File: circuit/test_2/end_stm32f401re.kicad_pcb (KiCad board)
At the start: 2 copper layers, 70 x 55.8 mm, 37 parts, among them J1 Micro_SD_Card_Det, J2 USB_B_Micro, U1 MAX98357_DAC, U2 STM32F401RETx, U3 AMS1117-3.3

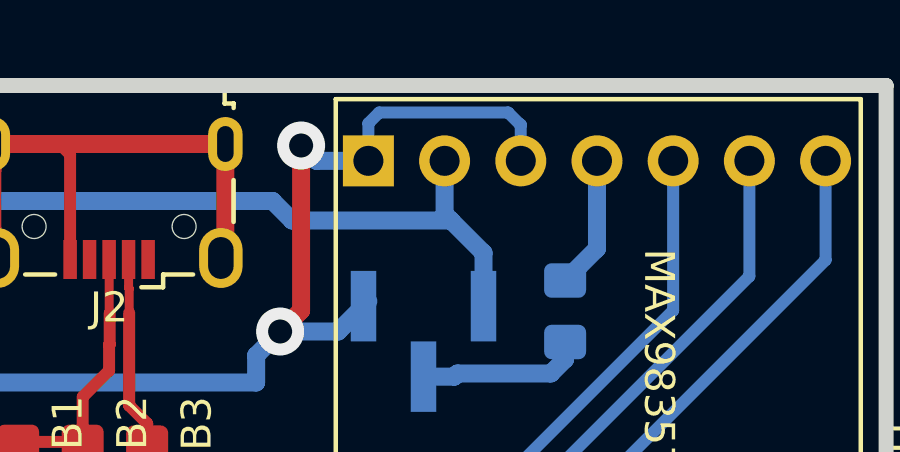
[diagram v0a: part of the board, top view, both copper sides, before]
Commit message: test 2 progress
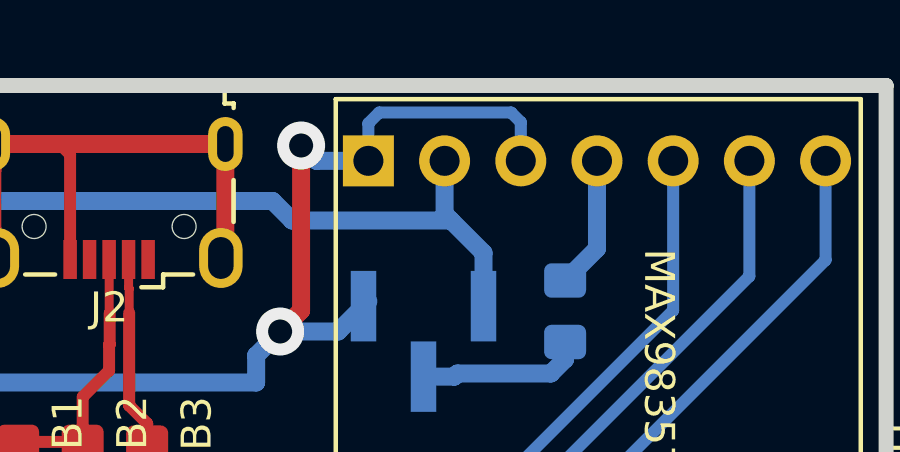
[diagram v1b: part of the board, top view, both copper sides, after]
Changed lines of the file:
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@@
     (thickness 1.6)
     (drawings 5)
-    (tracks 634)
+    (tracks 632)
     (zones 0)
     (modules 37)
@@
   (segment (start 128.644999 80.455001) (end 128.7 80.4) (width 0.6) (layer F.Cu) (net 16))
   (segment (start 123.395001 80.455001) (end 128.644999 80.455001) (width 0.6) (layer F.Cu) (net 16))
-  (segment (start 120.742111 36.261391) (end 121.103502 35.9) (width 0.4) (layer B.Cu) (net 16))
-  (segment (start 120.742111 37.511391) (end 120.742111 36.261391) (width 0.4) (layer B.Cu) (net 16))
-  (segment (start 121.103502 35.9) (end 125.4 35.9) (width 0.4) (layer B.Cu) (net 16))
-  (segment (start 125.4 35.9) (end 125.8 36.3) (width 0.4) (layer B.Cu) (net 16))
-  (segment (start 125.822111 36.30931) (end 125.822111 37.511391) (width 0.4) (layer B.Cu) (net 16))
-  (segment (start 125.812801 36.3) (end 125.822111 36.30931) (width 0.4) (layer B.Cu) (net 16))
-  (segment (start 125.8 36.3) (end 125.812801 36.3) (width 0.4) (layer B.Cu) (net 16))
   (via (at 114.4 82.6) (size 1.6) (drill 0.8) (layers F.Cu B.Cu) (net 16))
   (segment (start 113.1 81.3) (end 114.4 82.6) (width 0.6) (layer B.Cu) (net 16))
@@
   (segment (start 103.1 44.9) (end 107.4 44.9) (width 0.4) (layer F.Cu) (net 16))
   (segment (start 102.2 44) (end 103.1 44.9) (width 0.4) (layer F.Cu) (net 16))
+  (segment (start 120.742111 36.261391) (end 121.103502 35.9) (width 0.4) (layer B.Cu) (net 16))
+  (segment (start 120.742111 37.511391) (end 120.742111 36.261391) (width 0.4) (layer B.Cu) (net 16))
+  (segment (start 121.103502 35.9) (end 125.5 35.9) (width 0.4) (layer B.Cu) (net 16))
+  (segment (start 125.822111 36.222111) (end 125.822111 37.511391) (width 0.4) (layer B.Cu) (net 16))
+  (segment (start 125.5 35.9) (end 125.822111 36.222111) (width 0.4) (layer B.Cu) (net 16))
   (segment (start 105.03 56.005) (end 105.03 51.23) (width 0.3) (layer F.Cu) (net 17))
   (segment (start 105.03 51.23) (end 99.7 45.9) (width 0.3) (layer F.Cu) (net 17))
